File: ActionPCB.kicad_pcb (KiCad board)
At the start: 2 copper layers, 43 x 30 mm, 36 parts, among them P1 VCC, P10 GND, P11 SCL, P12 SDA, P13 CH1, P14 CH2, P15 CH3, P16 CH4, P2 GND, P3 SCL, P4 SDA, P5 CH1, P6 CH2, P7 CH3, P8 CH4, P9 VCC, U1 MPU-6050, U2 AMS1117-3.3

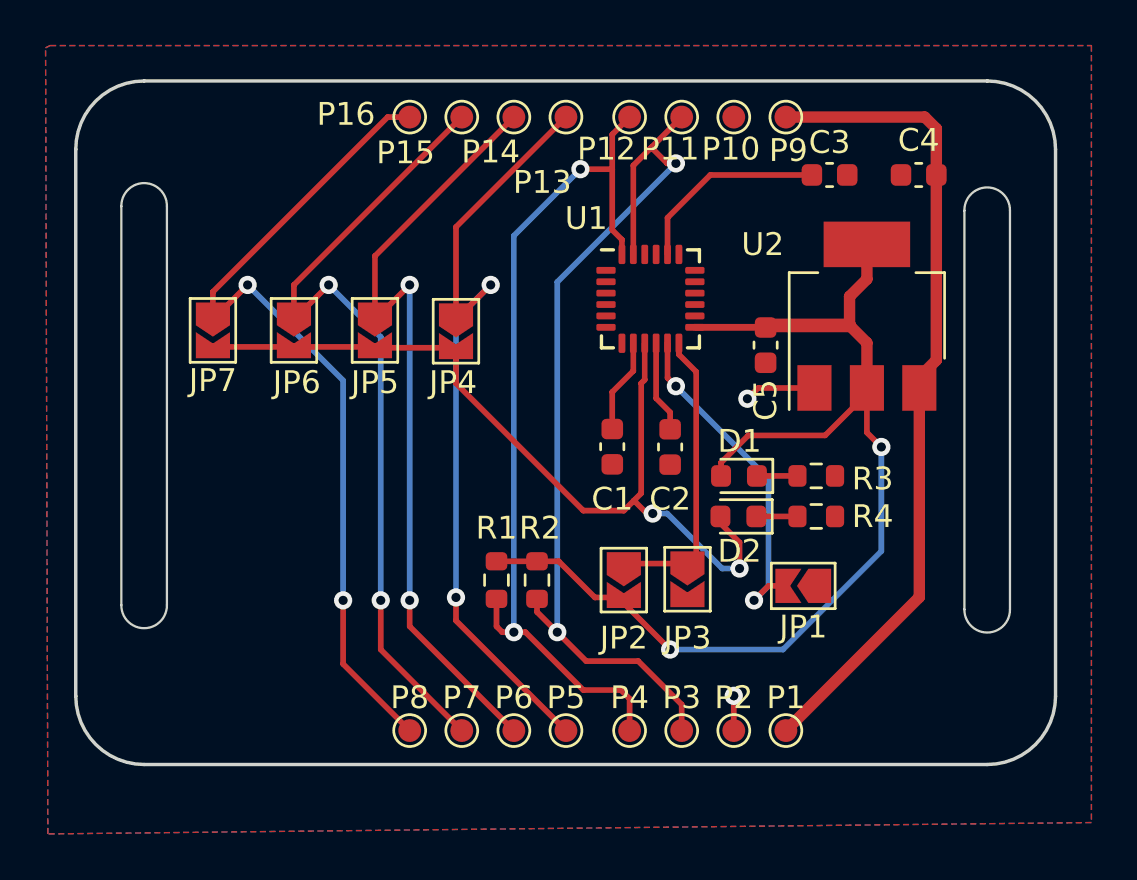
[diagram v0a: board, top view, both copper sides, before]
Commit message: Final board single
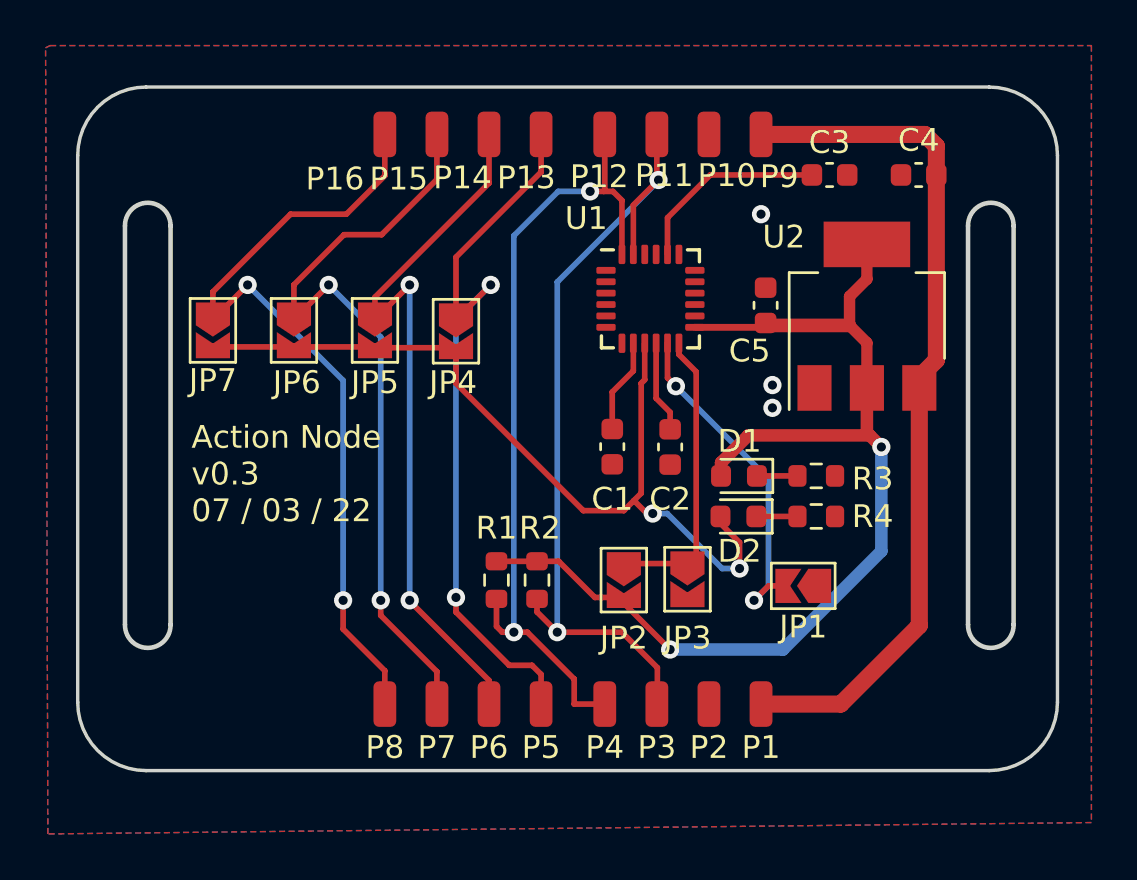
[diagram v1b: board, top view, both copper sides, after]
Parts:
- P1, P10, P11, P12, P13, P14, P15, P16, P2, P3, P4, P5, P6, P7, P8, P9: footprint TestPoint:TestPoint_Pad_D1.0mm -> Connector_Wire:SolderWirePad_1x01_SMD_1x2mm
- moved C5 1.75 mm to (131.7, 43.5), turned to 90 degrees
- moved P1 1.59 mm to (131.5, 61.0)
- moved P2 1.59 mm to (129.2, 61.0)
- moved P3 1.59 mm to (126.9, 61.0)
- moved P4 1.59 mm to (124.6, 61.0)
- moved P5 1.59 mm to (121.8, 61.0)
- moved P6 1.59 mm to (119.6, 61.0)
- moved P7 1.59 mm to (117.3, 61.0)
- moved P8 1.59 mm to (115.0, 61.0)
- moved P10 1.33 mm to (129.2, 36.0)
- moved P11 1.33 mm to (126.9, 36.0)
- moved P12 1.33 mm to (124.6, 36.0)
- moved P13 1.33 mm to (121.8, 36.0)
- moved P14 1.33 mm to (119.6, 36.0)
- moved P15 1.33 mm to (117.3, 36.0)
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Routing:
- net /SCL: track 40.8 -> 35.9 mm
- net GND: track 4.67 -> 0.00 mm, vias 2 -> 3
- net /SDA: track 39.2 -> 36.0 mm
- net /CH2: track 34.7 -> 31.8 mm
- net /CH1: track 34.9 -> 32.7 mm
- net /CH4: track 37.3 -> 35.4 mm
- net /CH3: track 35.7 -> 33.9 mm
- net VCC: track 36.0 -> 37.6 mm
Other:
- outline, holes or cut-outs redrawn
- board text added: "Action Node v0.3 07 / 03 / 22"
- board text added: "V G C D 1 2 3 4"
